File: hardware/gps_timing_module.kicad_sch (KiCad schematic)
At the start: 7 parts, among them J3 UART GPS, U9 LEA-M8T

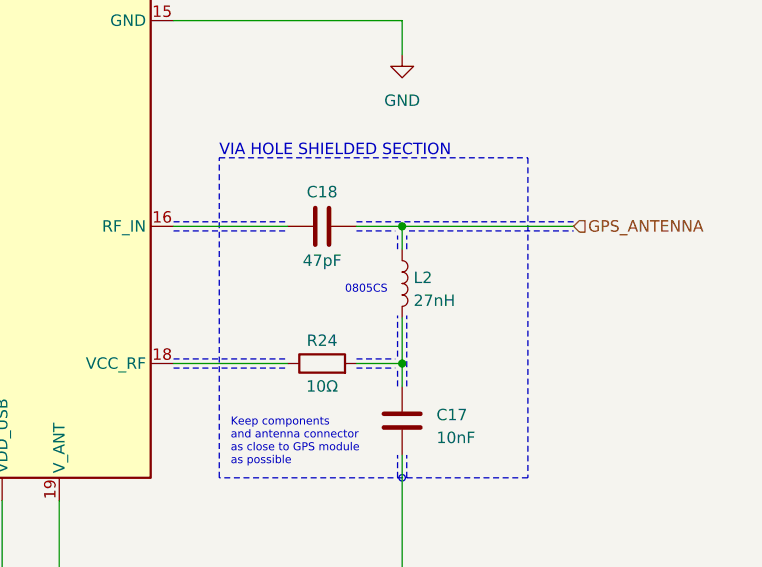
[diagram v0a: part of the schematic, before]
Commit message: Prepare v8 project for KiCAD version 9
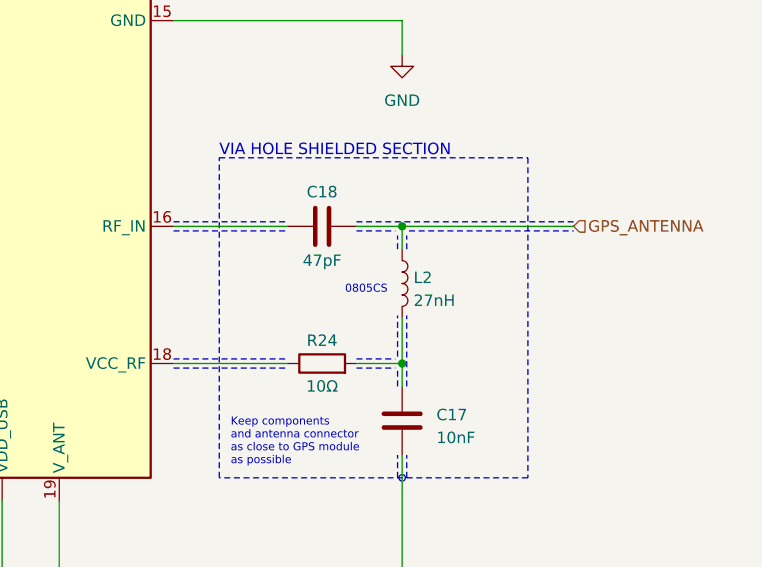
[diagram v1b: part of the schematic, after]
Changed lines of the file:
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@@
 (kicad_sch
-	(version 20231120)
+	(version 20250114)
 	(generator "eeschema")
-	(generator_version "8.0")
+	(generator_version "9.0")
 	(paper "A4")
 	(title_block
@@
 		(comment 1 "GPS timing module")
 	)
+	(circle
+		(center 189.23 139.7)
+		(radius 0.3592)
+		(stroke
+			(width -0.0001)
+			(type default)
+		)
+		(fill
+			(type color)
+			(color 0 0 132 1)
+		)
+	)
+	(rectangle
+		(start 168.91 104.14)
+		(end 203.2 139.7)
+		(stroke
+			(width 0)
+			(type dash)
+		)
+		(fill
+			(type none)
+		)
+	)
+	(text "SAFEBOOT"
+		(exclude_from_sim no)
+		(at 93.345 66.675 0)
+		(effects
+			(font
+				(size 0.889 0.889)
+			)
+			(justify right bottom)
+		)
+	)
+	(text "0805CS"
+		(exclude_from_sim no)
+		(at 182.88 119.38 0)
+		(effects
+			(font
+				(size 0.889 0.889)
+			)
+			(justify left bottom)
+		)
+	)
+	(text "Keep components\nand antenna connector\nas close to GPS module\nas possible"
+		(exclude_from_sim no)
+		(at 170.18 138.43 0)
+		(effects
+			(font
+				(size 0.889 0.889)
+			)
+			(justify left bottom)
+		)
+	)
+	(text "D_SEL n/c to enable\nUART on pin 3 and 4\nand I^{2}C on 1 and 2"
+		(exclude_from_sim no)
+		(at 90.17 97.155 0)
+		(effects
+			(font
+				(size 0.889 0.889)
+			)
+			(justify left bottom)
+		)
+	)
+	(text "RESET"
+		(exclude_from_sim no)
+		(at 93.345 69.215 0)
+		(effects
+			(font
+				(size 0.889 0.889)
+			)
+			(justify right bottom)
+		)
+	)
+	(text "VIA HOLE SHIELDED SECTION"
+		(exclude_from_sim no)
+		(at 168.91 104.14 0)
+		(effects
+			(font
+				(size 1.27 1.27)
+			)
+			(justify left bottom)
+		)
+	)
+	(text "RXD"
+		(exclude_from_sim no)
+		(at 93.345 64.135 0)
+		(effects
+			(font
+				(size 0.889 0.889)
+			)
+			(justify right bottom)
+		)
+	)
+	(text "GND"
+		(exclude_from_sim no)
+		(at 93.345 71.755 0)
+		(effects
+			(font
+				(size 0.889 0.889)
+			)
+			(justify right bottom)
+		)
+	)
+	(text "TXD"
+		(exclude_from_sim no)
+		(at 93.345 61.595 0)
+		(effects
+			(font
+				(size 0.889 0.889)
+			)
+			(justify right bottom)
+		)
+	)
+	(text "+3.3V"
+		(exclude_from_sim no)
+		(at 93.345 59.055 0)
+		(effects
+			(font
+				(size 0.889 0.889)
+			)
+			(justify right bottom)
+		)
+	)
 	(junction
 		(at 107.95 132.08)
@@
 		)
 	)
-	(circle
-		(center 189.23 139.7)
-		(radius 0.3592)
-		(stroke
-			(width -0.0001)
-			(type default)
-		)
-		(fill
-			(type color)
-			(color 0 0 132 1)
-		)
-	)
-	(rectangle
-		(start 168.91 104.14)
-		(end 203.2 139.7)
-		(stroke
-			(width 0)
-			(type dash)
-		)
-		(fill
-			(type none)
-		)
-	)
-	(text "SAFEBOOT"
-		(exclude_from_sim no)
-		(at 93.345 66.675 0)
-		(effects
-			(font
-				(size 0.889 0.889)
-			)
-			(justify right bottom)
-		)
-	)
-	(text "0805CS"
-		(exclude_from_sim no)
-		(at 182.88 119.38 0)
-		(effects
-			(font
-				(size 0.889 0.889)
-			)
-			(justify left bottom)
-		)
-	)
-	(text "Keep components\nand antenna connector\nas close to GPS module\nas possible"
-		(exclude_from_sim no)
-		(at 170.18 138.43 0)
-		(effects
-			(font
-				(size 0.889 0.889)
-			)
-			(justify left bottom)
-		)
-	)
-	(text "D_SEL n/c to enable\nUART on pin 3 and 4\nand I^{2}C on 1 and 2"
-		(exclude_from_sim no)
-		(at 90.17 97.155 0)
-		(effects
-			(font
-				(size 0.889 0.889)
-			)
-			(justify left bottom)
-		)
-	)
-	(text "RESET"
-		(exclude_from_sim no)
-		(at 93.345 69.215 0)
-		(effects
-			(font
-				(size 0.889 0.889)
-			)
-			(justify right bottom)
-		)
-	)
-	(text "VIA HOLE SHIELDED SECTION"
-		(exclude_from_sim no)
-		(at 168.91 104.14 0)
-		(effects
-			(font
-				(size 1.27 1.27)
-			)
-			(justify left bottom)
-		)
-	)
-	(text "RXD"
-		(exclude_from_sim no)
-		(at 93.345 64.135 0)
-		(effects
-			(font
-				(size 0.889 0.889)
-			)
-			(justify right bottom)
-		)
-	)
-	(text "GND"
-		(exclude_from_sim no)
-		(at 93.345 71.755 0)
-		(effects
-			(font
-				(size 0.889 0.889)
-			)
-			(justify right bottom)
-		)
-	)
-	(text "TXD"
-		(exclude_from_sim no)
-		(at 93.345 61.595 0)
-		(effects
-			(font
-				(size 0.889 0.889)
-			)
-			(justify right bottom)
-		)
-	)
-	(text "+3.3V"
-		(exclude_from_sim no)
-		(at 93.345 59.055 0)
-		(effects
-			(font
-				(size 0.889 0.889)
-			)
-			(justify right bottom)
-		)
-	)
 	(hierarchical_label "GPS_TIMEPULSE"
 		(shape output)
 		(at 208.28 63.5 0)
-		(fields_autoplaced yes)
 		(effects
 			(font
@@
 		(shape input)
 		(at 107.95 119.38 180)
-		(fields_autoplaced yes)
 		(effects
 			(font
@@
 		(shape input)
 		(at 208.28 111.76 0)
-		(fields_autoplaced yes)
 		(effects
 			(font
@@
 		(shape bidirectional)
 		(at 107.95 116.84 180)
-		(fields_autoplaced yes)
-		(effects
-			(font
+		(effects
+			(font
